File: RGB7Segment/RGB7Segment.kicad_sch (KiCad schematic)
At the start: 21 parts, among them J1 Conn_01x02_Socket, J2 Conn_01x02_Socket

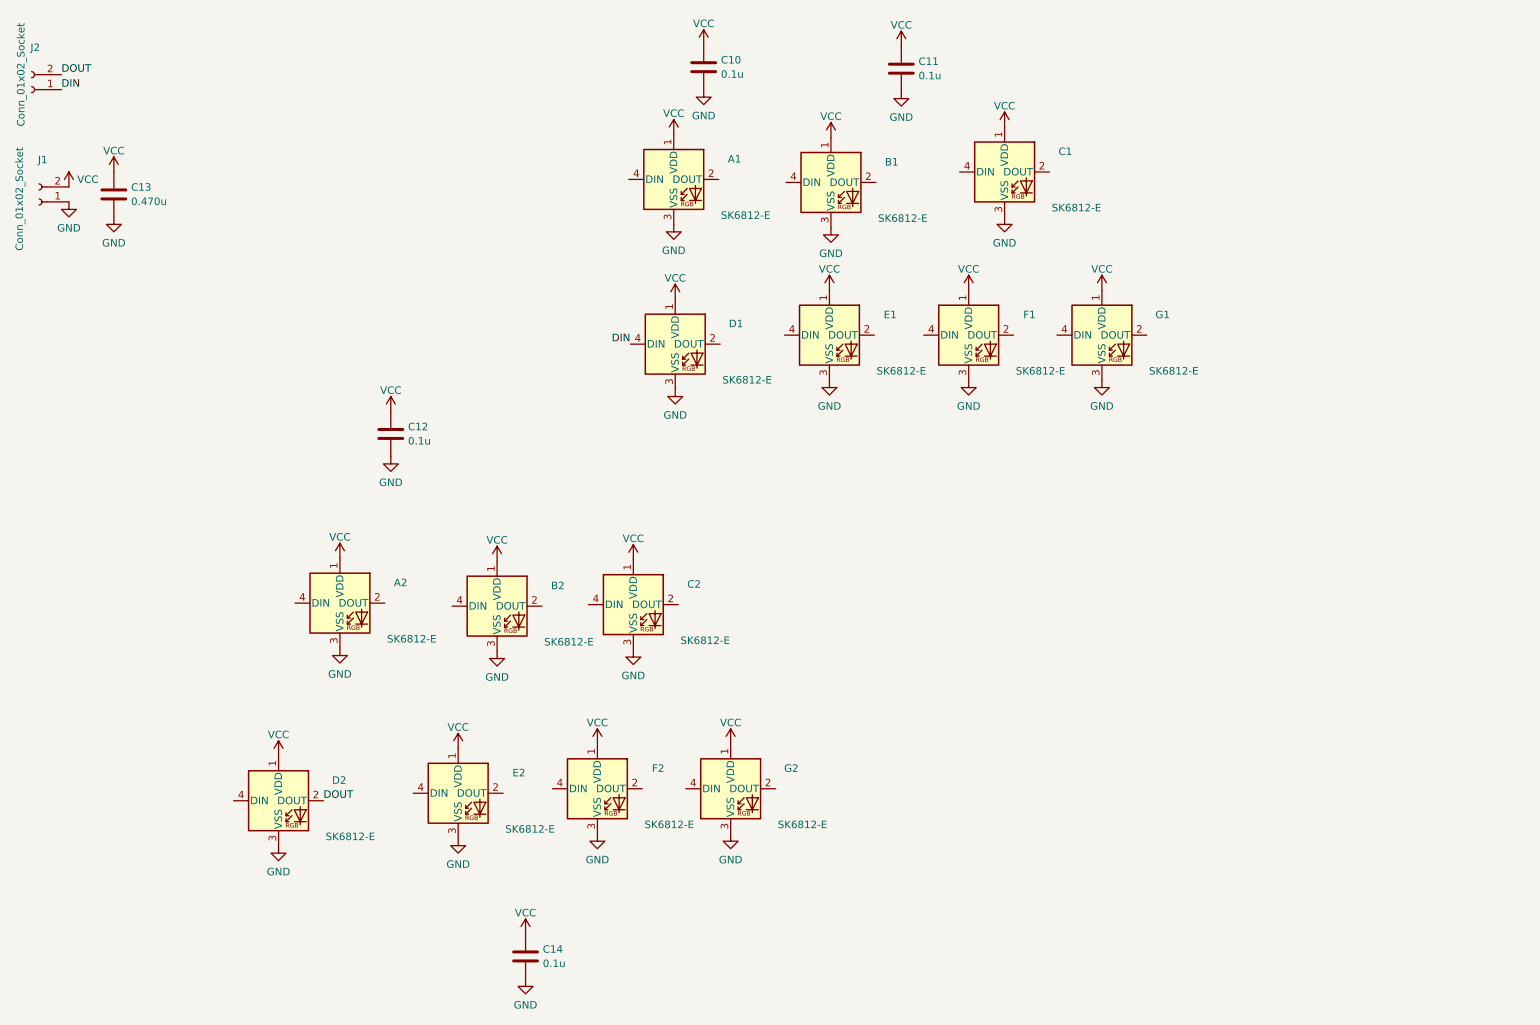
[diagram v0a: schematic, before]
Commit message: New Pass of RGB 7 Segment
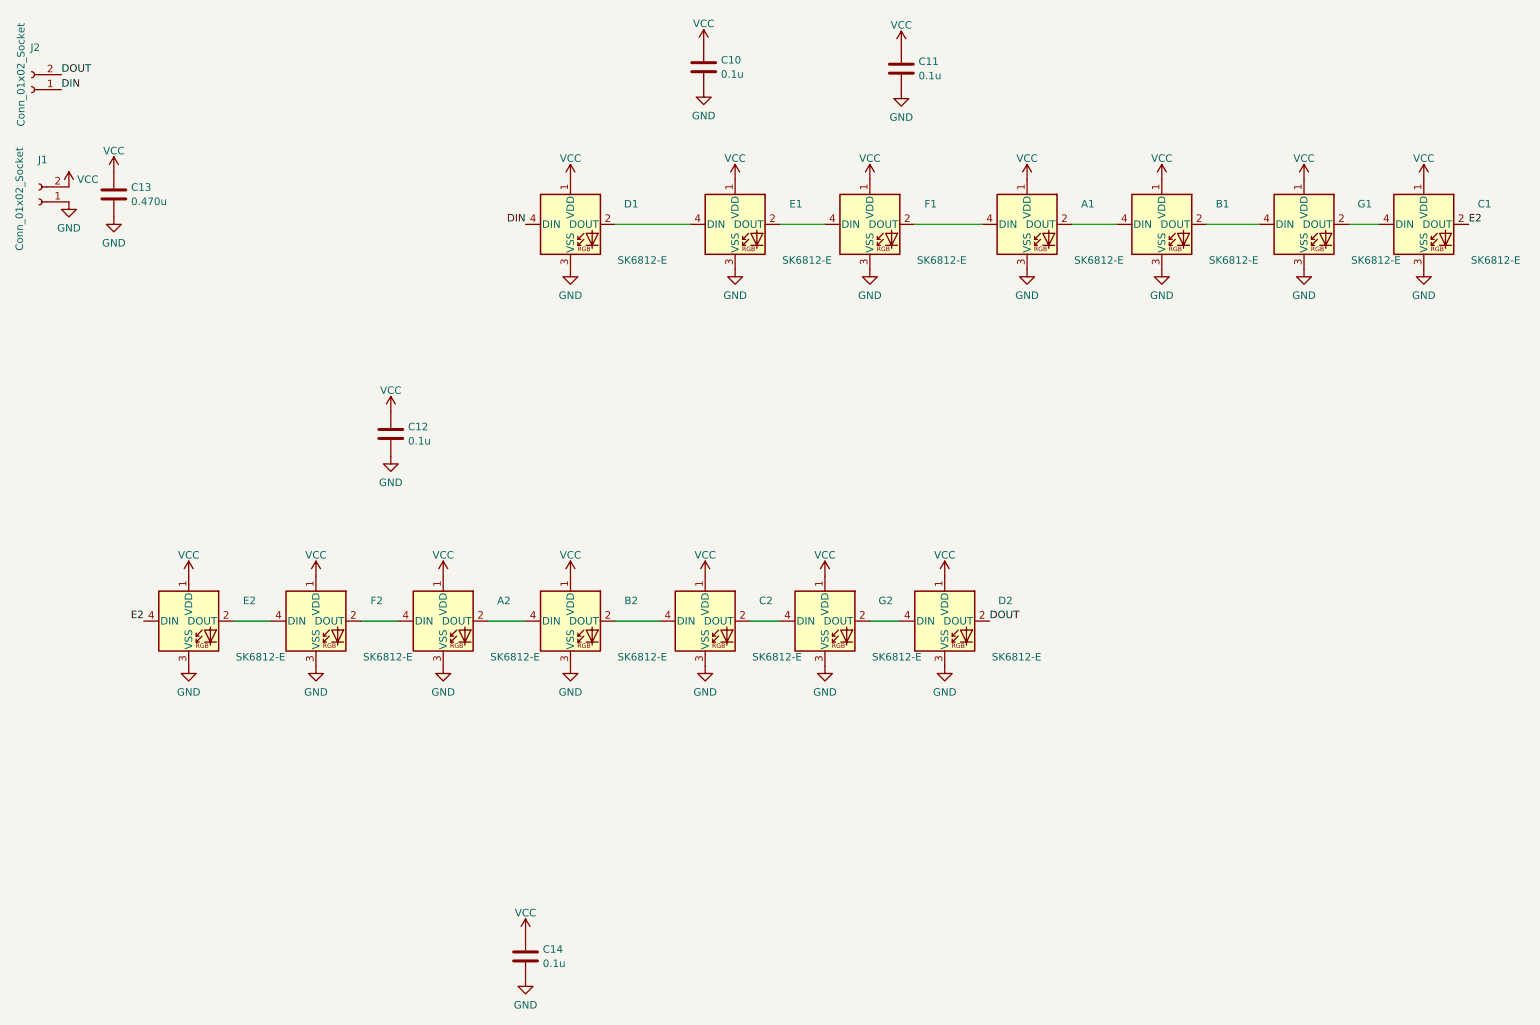
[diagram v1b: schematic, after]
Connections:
- net E2: now reaches C1.2 (DOUT)
- net E2: now also E2.4 (DIN)
- net at C1.4 (DIN): now also G1.2 (DOUT)
- net at A2.2 (DOUT): now also B2.4 (DIN)
- net at A2.4 (DIN): now also F2.2 (DOUT)
- net at B1.2 (DOUT): now also G1.4 (DIN)
- net at B1.4 (DIN): now also A1.2 (DOUT)
- net at C2.2 (DOUT): now also G2.4 (DIN)
- net at C2.4 (DIN): now also B2.2 (DOUT)
- net at D2.4 (DIN): now also G2.2 (DOUT)
- net at F1.2 (DOUT): now also A1.4 (DIN)
- net at F1.4 (DIN): now also E1.2 (DOUT)
- net at E2.2 (DOUT): now also F2.4 (DIN)
- net at E1.4 (DIN): now also D1.2 (DOUT)
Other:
- moved on the sheet: A1, A2, B1, B2, C1, C2, D1, D2, E1, E2, F1, F2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
